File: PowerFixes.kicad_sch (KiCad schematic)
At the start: 6 parts, among them SW10 L103011MS02Q, U30 LT1175-5_SOT223

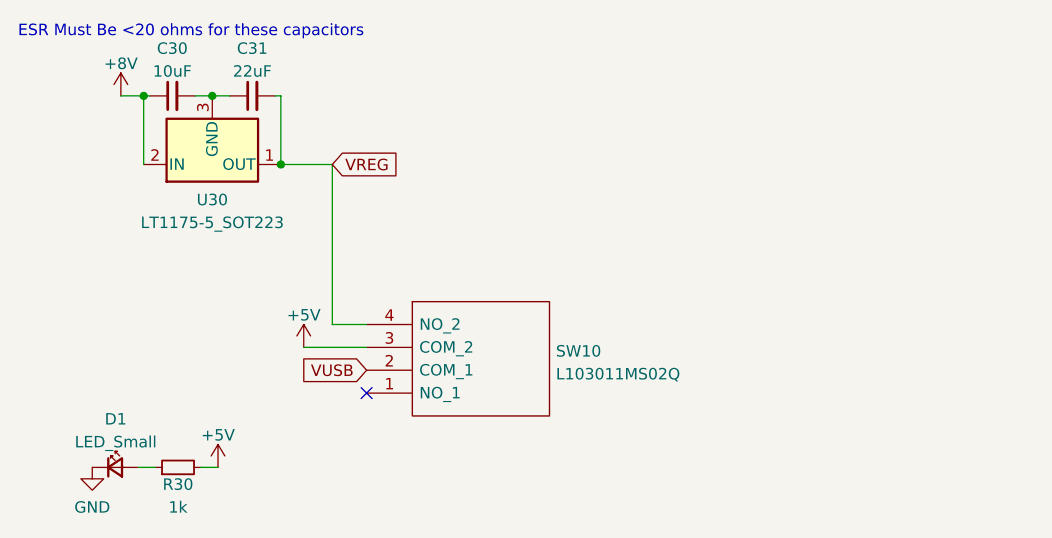
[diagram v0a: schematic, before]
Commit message: Pushing PCB
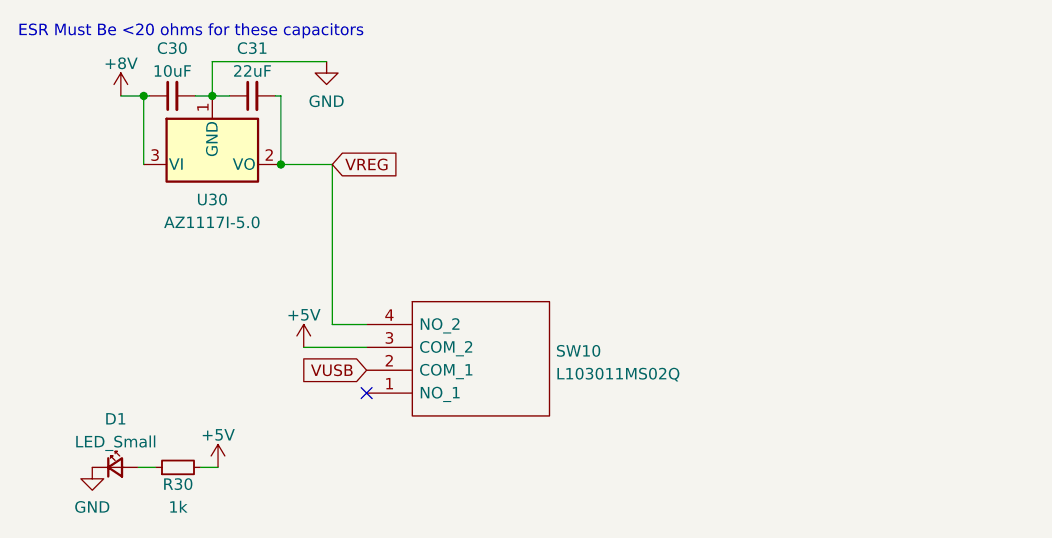
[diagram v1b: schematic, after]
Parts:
- removed U30: LT1175-5_SOT223, Package_TO_SOT_SMD:SOT-223-3_TabPin2, symbol Regulator_Linear:LT1175-5_SOT223
- added U30: AZ1117I-5.0, Package_TO_SOT_SMD:SOT-223-3_TabPin2, symbol Regulator_Linear:NCP1117-12_SOT223
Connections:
- net +8V: now also U30.3 (VI)
- net GND: now also C30.2, C31.1, U30.1 (GND)
- net VREG: now also U30.2 (VO)
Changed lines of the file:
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@@
+    (stroke (width 0) (type default) (color 0 0 0 0))
+  )
+  (wire (pts (xy 38.1 25.4) (xy 38.1 21.59))
     (stroke (width 0) (type default) (color 0 0 0 0))
   )
   (wire (pts (xy 30.48 25.4) (xy 31.115 25.4))
+    (stroke (width 0) (type default) (color 0 0 0 0))
+  )
+  (wire (pts (xy 38.1 21.59) (xy 50.8 21.59))
     (stroke (width 0) (type default) (color 0 0 0 0))
   )
@@
     (pin "2")
   )
-  (symbol (lib_id "Regulator_Linear:LT1175-5_SOT223") (at 38.1 33.02 0) (unit 1)
-    (in_bom yes) (on_board yes) (fields_autoplaced)
-    (property "Reference" "U30" (id 0) (at 38.1 36.9554 0))
-    (property "Value" "LT1175-5_SOT223" (id 1) (at 38.1 39.4923 0))
-    (property "Footprint" "Package_TO_SOT_SMD:SOT-223-3_TabPin2" (id 2) (at 38.1 38.1 0)
-      (effects (font (size 1.27 1.27)) hide)
-    )
-    (property "Datasheet" "https://www.analog.com/media/en/technical-documentation/data-sheets/1175ff.pdf" (id 3) (at 38.735 33.02 0)
-      (effects (font (size 1.27 1.27)) hide)
-    )
-    (pin "1")
-    (pin "2")
-    (pin "3")
-  )
   (symbol (lib_id "power:+5V") (at 48.26 53.34 0) (unit 1)
     (in_bom yes) (on_board yes) (fields_autoplaced)
@@
     (pin "1")
   )
+  (symbol (lib_id "power:GND") (at 50.8 21.59 0) (unit 1)
+    (in_bom yes) (on_board yes) (fields_autoplaced)
+    (property "Reference" "#PWR0152" (id 0) (at 50.8 27.94 0)
+      (effects (font (size 1.27 1.27)) hide)
+    )
+    (property "Value" "GND" (id 1) (at 50.8 26.0334 0))
+    (property "Footprint" "" (id 2) (at 50.8 21.59 0)
+      (effects (font (size 1.27 1.27)) hide)
+    )
+    (property "Datasheet" "" (id 3) (at 50.8 21.59 0)
+      (effects (font (size 1.27 1.27)) hide)
+    )
+    (pin "1")
+  )
+  (symbol (lib_id "Regulator_Linear:NCP1117-12_SOT223") (at 38.1 33.02 0) (mirror x) (unit 1)
+    (in_bom yes) (on_board yes) (fields_autoplaced)
+    (property "Reference" "U30" (id 0) (at 38.1 36.9554 0))
+    (property "Value" "AZ1117I-5.0" (id 1) (at 38.1 39.4923 0))
+    (property "Footprint" "Package_TO_SOT_SMD:SOT-223-3_TabPin2" (id 2) (at 38.1 38.1 0)
+      (effects (font (size 1.27 1.27)) hide)
+    )
+    (property "Datasheet" "http://www.onsemi.com/pub_link/Collateral/NCP1117-D.PDF" (id 3) (at 40.64 26.67 0)
+      (effects (font (size 1.27 1.27)) hide)
+    )
+    (pin "1")
+    (pin "2")
+    (pin "3")
+  )
   (symbol (lib_id "Device:R_Small") (at 34.29 66.675 90) (unit 1)

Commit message: Changes... James Changes
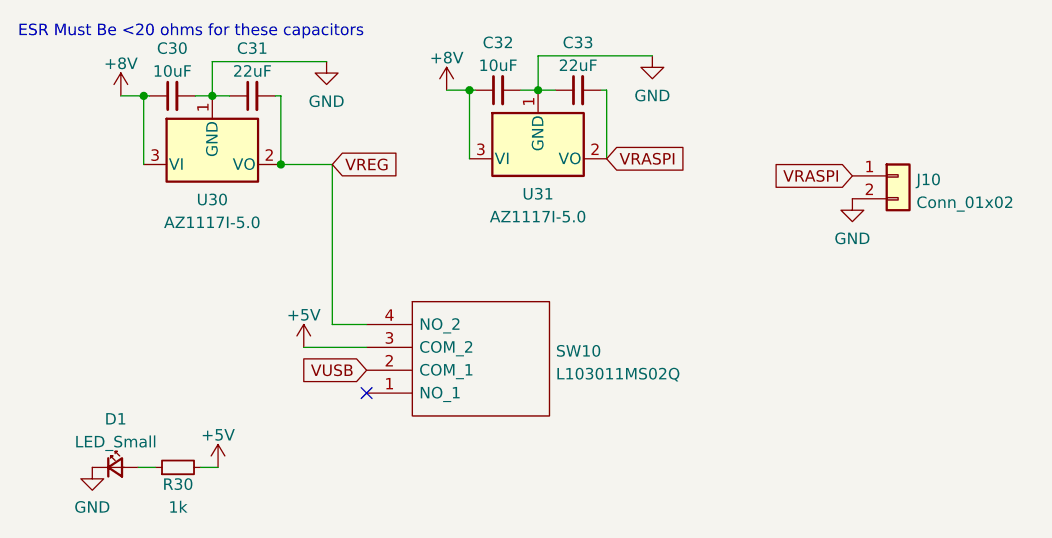
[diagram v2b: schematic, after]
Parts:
- added C32: 10uF, Capacitor_SMD:C_0805_2012Metric, symbol Device:C_Small
- added C33: 22uF, Capacitor_SMD:C_0805_2012Metric, symbol Device:C_Small
- added J10: Conn_01x02, CustomFootprints:POWER_TERM, symbol Connector_Generic:Conn_01x02
- added U31: AZ1117I-5.0, Package_TO_SOT_SMD:SOT-223-3_TabPin2, symbol Regulator_Linear:NCP1117-12_SOT223
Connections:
- net +8V: now also C32.1, U31.3 (VI)
- net GND: now also C32.2, C33.1, J10.2 (Pin_2), U31.1 (GND)
- new net VRASPI: C33.2, J10.1 (Pin_1), U31.2 (VO)
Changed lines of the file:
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@@
   (junction (at 45.72 33.02) (diameter 0) (color 0 0 0 0)
   )
+  (junction (at 66.675 24.765) (diameter 0) (color 0 0 0 0)
+  )
   (junction (at 30.48 25.4) (diameter 0) (color 0 0 0 0)
+  )
+  (junction (at 74.295 24.765) (diameter 0) (color 0 0 0 0)
   )
   (junction (at 38.1 25.4) (diameter 0) (color 0 0 0 0)
@@
     (stroke (width 0) (type default) (color 0 0 0 0))
   )
+  (wire (pts (xy 81.915 24.765) (xy 81.915 32.385))
+    (stroke (width 0) (type default) (color 0 0 0 0))
+  )
+  (wire (pts (xy 64.135 24.765) (xy 66.675 24.765))
+    (stroke (width 0) (type default) (color 0 0 0 0))
+  )
   (wire (pts (xy 48.26 53.34) (xy 55.245 53.34))
     (stroke (width 0) (type default) (color 0 0 0 0))
   )
+  (wire (pts (xy 74.295 20.955) (xy 86.995 20.955))
+    (stroke (width 0) (type default) (color 0 0 0 0))
+  )
   (wire (pts (xy 55.245 50.8) (xy 51.435 50.8))
     (stroke (width 0) (type default) (color 0 0 0 0))
@@
     (stroke (width 0) (type default) (color 0 0 0 0))
   )
+  (wire (pts (xy 72.39 24.765) (xy 74.295 24.765))
+    (stroke (width 0) (type default) (color 0 0 0 0))
+  )
   (wire (pts (xy 45.085 25.4) (xy 45.72 25.4))
     (stroke (width 0) (type default) (color 0 0 0 0))
@@
     (stroke (width 0) (type default) (color 0 0 0 0))
   )
+  (wire (pts (xy 74.295 24.765) (xy 76.2 24.765))
+    (stroke (width 0) (type default) (color 0 0 0 0))
+  )
   (wire (pts (xy 38.1 25.4) (xy 38.1 21.59))
     (stroke (width 0) (type default) (color 0 0 0 0))
   )
+  (wire (pts (xy 66.675 24.765) (xy 66.675 32.385))
+    (stroke (width 0) (type default) (color 0 0 0 0))
+  )
   (wire (pts (xy 30.48 25.4) (xy 31.115 25.4))
     (stroke (width 0) (type default) (color 0 0 0 0))
   )
+  (wire (pts (xy 66.675 24.765) (xy 67.31 24.765))
+    (stroke (width 0) (type default) (color 0 0 0 0))
+  )
+  (wire (pts (xy 74.295 24.765) (xy 74.295 20.955))
+    (stroke (width 0) (type default) (color 0 0 0 0))
+  )
   (wire (pts (xy 38.1 21.59) (xy 50.8 21.59))
+    (stroke (width 0) (type default) (color 0 0 0 0))
+  )
+  (wire (pts (xy 81.28 24.765) (xy 81.915 24.765))
     (stroke (width 0) (type default) (color 0 0 0 0))
   )
@@
     (property "Intersheet References" "${INTERSHEET_REFS}" (id 0) (at 58.6257 32.9406 0)
       (effects (font (size 1.27 1.27)) (justify left) hide)
+    )
+  )
+  (global_label "VRASPI" (shape input) (at 81.915 32.385 0) (fields_autoplaced)
+    (effects (font (size 1.27 1.27)) (justify left))
+    (property "Intersheet References" "${INTERSHEET_REFS}" (id 0) (at 90.8595 32.3056 0)
+      (effects (font (size 1.27 1.27)) (justify left) hide)
+    )
+  )
+  (global_label "VRASPI" (shape input) (at 109.22 34.29 180) (fields_autoplaced)
+    (effects (font (size 1.27 1.27)) (justify right))
+    (property "Intersheet References" "${INTERSHEET_REFS}" (id 0) (at 100.2755 34.2106 0)
+      (effects (font (size 1.27 1.27)) (justify right) hide)
     )
   )
@@
     (pin "1")
     (pin "2")
+  )
+  (symbol (lib_id "Device:C_Small") (at 69.85 24.765 90) (unit 1)
+    (in_bom yes) (on_board yes)
+    (property "Reference" "C32" (id 0) (at 69.8563 19.5031 90))
+    (property "Value" "10uF" (id 1) (at 69.8563 22.04 90))
+    (property "Footprint" "Capacitor_SMD:C_0805_2012Metric" (id 2) (at 69.85 24.765 0)
+      (effects (font (size 1.27 1.27)) hide)
+    )
+    (property "Datasheet" "~" (id 3) (at 69.85 24.765 0)
+      (effects (font (size 1.27 1.27)) hide)
+    )
+    (pin "1")
+    (pin "2")
+  )
+  (symbol (lib_id "power:GND") (at 50.8 21.59 0) (unit 1)
+    (in_bom yes) (on_board yes) (fields_autoplaced)
+    (property "Reference" "#PWR0156" (id 0) (at 50.8 27.94 0)
+      (effects (font (size 1.27 1.27)) hide)
+    )
+    (property "Value" "GND" (id 1) (at 50.8 26.0334 0))
+    (property "Footprint" "" (id 2) (at 50.8 21.59 0)
+      (effects (font (size 1.27 1.27)) hide)
+    )
+    (property "Datasheet" "" (id 3) (at 50.8 21.59 0)
+      (effects (font (size 1.27 1.27)) hide)
+    )
+    (pin "1")
   )
   (symbol (lib_id "Device:C_Small") (at 33.655 25.4 90) (unit 1)
@@
     (pin "1")
   )
+  (symbol (lib_id "Regulator_Linear:NCP1117-12_SOT223") (at 74.295 32.385 0) (mirror x) (unit 1)
+    (in_bom yes) (on_board yes) (fields_autoplaced)
+    (property "Reference" "U31" (id 0) (at 74.295 36.3204 0))
+    (property "Value" "AZ1117I-5.0" (id 1) (at 74.295 38.8573 0))
+    (property "Footprint" "Package_TO_SOT_SMD:SOT-223-3_TabPin2" (id 2) (at 74.295 37.465 0)
+      (effects (font (size 1.27 1.27)) hide)
+    )
+    (property "Datasheet" "http://www.onsemi.com/pub_link/Collateral/NCP1117-D.PDF" (id 3) (at 76.835 26.035 0)
+      (effects (font (size 1.27 1.27)) hide)
+    )
+    (pin "1")
+    (pin "2")
+    (pin "3")
+  )
   (symbol (lib_id "power:+5V") (at 38.735 66.675 0) (unit 1)
     (in_bom yes) (on_board yes) (fields_autoplaced)
@@
     (pin "1")
   )
-  (symbol (lib_id "power:GND") (at 50.8 21.59 0) (unit 1)
-    (in_bom yes) (on_board yes) (fields_autoplaced)
-    (property "Reference" "#PWR0152" (id 0) (at 50.8 27.94 0)
-      (effects (font (size 1.27 1.27)) hide)
-    )
-    (property "Value" "GND" (id 1) (at 50.8 26.0334 0))
-    (property "Footprint" "" (id 2) (at 50.8 21.59 0)
-      (effects (font (size 1.27 1.27)) hide)
-    )
-    (property "Datasheet" "" (id 3) (at 50.8 21.59 0)
-      (effects (font (size 1.27 1.27)) hide)
-    )
-    (pin "1")
+  (symbol (lib_id "power:GND") (at 109.22 36.83 0) (unit 1)
+    (in_bom yes) (on_board yes) (fields_autoplaced)
+    (property "Reference" "#PWR0157" (id 0) (at 109.22 43.18 0)
+      (effects (font (size 1.27 1.27)) hide)
+    )
+    (property "Value" "GND" (id 1) (at 109.22 41.2734 0))
+    (property "Footprint" "" (id 2) (at 109.22 36.83 0)
+      (effects (font (size 1.27 1.27)) hide)
+    )
+    (property "Datasheet" "" (id 3) (at 109.22 36.83 0)
+      (effects (font (size 1.27 1.27)) hide)
+    )
+    (pin "1")
+  )
+  (symbol (lib_id "power:GND") (at 86.995 20.955 0) (unit 1)
+    (in_bom yes) (on_board yes) (fields_autoplaced)
+    (property "Reference" "#PWR0152" (id 0) (at 86.995 27.305 0)
+      (effects (font (size 1.27 1.27)) hide)
+    )
+    (property "Value" "GND" (id 1) (at 86.995 25.3984 0))
+    (property "Footprint" "" (id 2) (at 86.995 20.955 0)
+      (effects (font (size 1.27 1.27)) hide)
+    )
+    (property "Datasheet" "" (id 3) (at 86.995 20.955 0)
+      (effects (font (size 1.27 1.27)) hide)
+    )
+    (pin "1")
+  )
+  (symbol (lib_id "Device:C_Small") (at 78.74 24.765 90) (unit 1)
+    (in_bom yes) (on_board yes) (fields_autoplaced)
+    (property "Reference" "C33" (id 0) (at 78.7463 19.5031 90))
+    (property "Value" "22uF" (id 1) (at 78.7463 22.04 90))
+    (property "Footprint" "Capacitor_SMD:C_0805_2012Metric" (id 2) (at 78.74 24.765 0)
+      (effects (font (size 1.27 1.27)) hide)
+    )
+    (property "Datasheet" "~" (id 3) (at 78.74 24.765 0)
+      (effects (font (size 1.27 1.27)) hide)
+    )
+    (pin "1")
+    (pin "2")
   )
   (symbol (lib_id "Regulator_Linear:NCP1117-12_SOT223") (at 38.1 33.02 0) (mirror x) (unit 1)
@@
     (pin "2")
     (pin "3")
+  )
+  (symbol (lib_id "power:+8V") (at 64.135 24.765 0) (unit 1)
+    (in_bom yes) (on_board yes) (fields_autoplaced)
+    (property "Reference" "#PWR0155" (id 0) (at 64.135 28.575 0)
+      (effects (font (size 1.27 1.27)) hide)
+    )
+    (property "Value" "+8V" (id 1) (at 64.135 21.1892 0))
+    (property "Footprint" "" (id 2) (at 64.135 24.765 0)
+      (effects (font (size 1.27 1.27)) hide)
+    )
+    (property "Datasheet" "" (id 3) (at 64.135 24.765 0)
+      (effects (font (size 1.27 1.27)) hide)
+    )
+    (pin "1")
   )
   (symbol (lib_id "Device:R_Small") (at 34.29 66.675 90) (unit 1)
@@
       (effects (font (size 1.27 1.27)) hide)
     )
+    (pin "1")
+    (pin "2")
+  )
+  (symbol (lib_id "Connector_Generic:Conn_01x02") (at 114.3 34.29 0) (unit 1)
+    (in_bom yes) (on_board yes) (fields_autoplaced)
+    (property "Reference" "J10" (id 0) (at 116.332 34.7253 0)
+      (effects (font (size 1.27 1.27)) (justify left))
+    )
+    (property "Value" "Conn_01x02" (id 1) (at 116.332 37.2622 0)
+      (effects (font (size 1.27 1.27)) (justify left))
+    )
+    (property "Footprint" "CustomFootprints:POWER_TERM" (id 2) (at 114.3 34.29 0)
+      (effects (font (size 1.27 1.27)) hide)
+    )
+    (property "Datasheet" "~" (id 3) (at 114.3 34.29 0)
+      (effects (font (size 1.27 1.27)) hide)
+    )
